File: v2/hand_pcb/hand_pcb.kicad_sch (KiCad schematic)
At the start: 60 parts, among them J1 Screw_Terminal_01x10, J10 8P8C, J2 Conn_01x08, J3 Conn_01x08, J4 Conn_01x02, J5 Conn_01x02, J9 Conn_02x02_Top_Bottom, M1 Motor_Servo_FB, M10 Motor_Servo_FB, M2 Motor_Servo_FB, M3 Motor_Servo_FB, M4 Motor_Servo_FB, M5 Motor_Servo_FB, M6 Motor_Servo_FB, M7 Motor_Servo_FB, M8 Motor_Servo_FB, M9 Motor_Servo_FB, Q1 Q_NMOS_GDS, Q2 Q_NMOS_GDS, Q3 Q_NMOS_GDS, Q4 Q_NMOS_GDS, Q5 Q_NMOS_GDS, U1 PCA9685PW, U2 MCP23017_SP, U4 ADS7830, U5 ADS7830

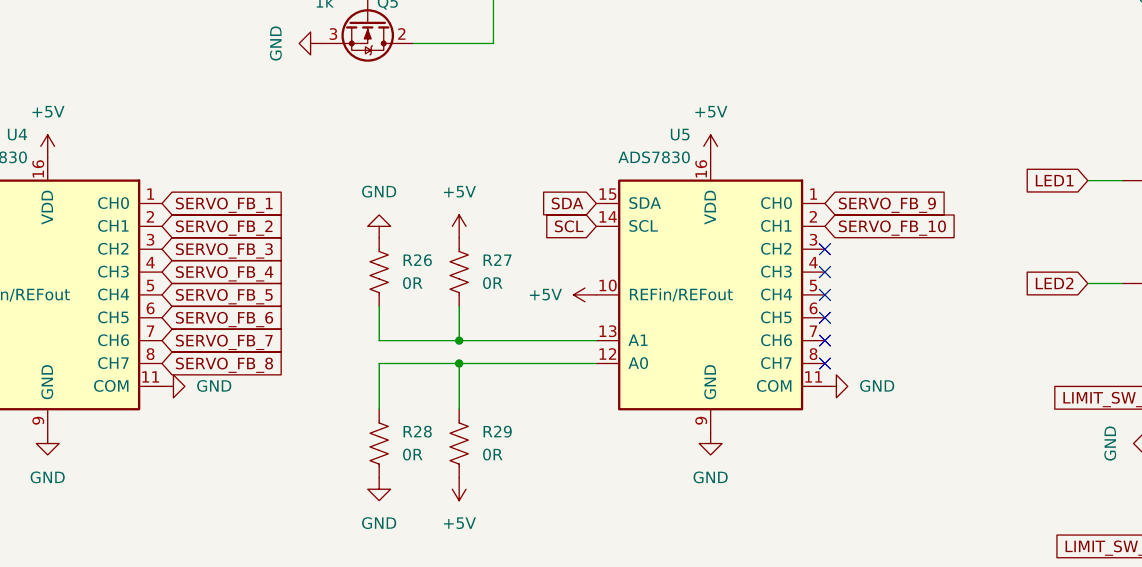
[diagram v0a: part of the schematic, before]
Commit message: Doing stuff
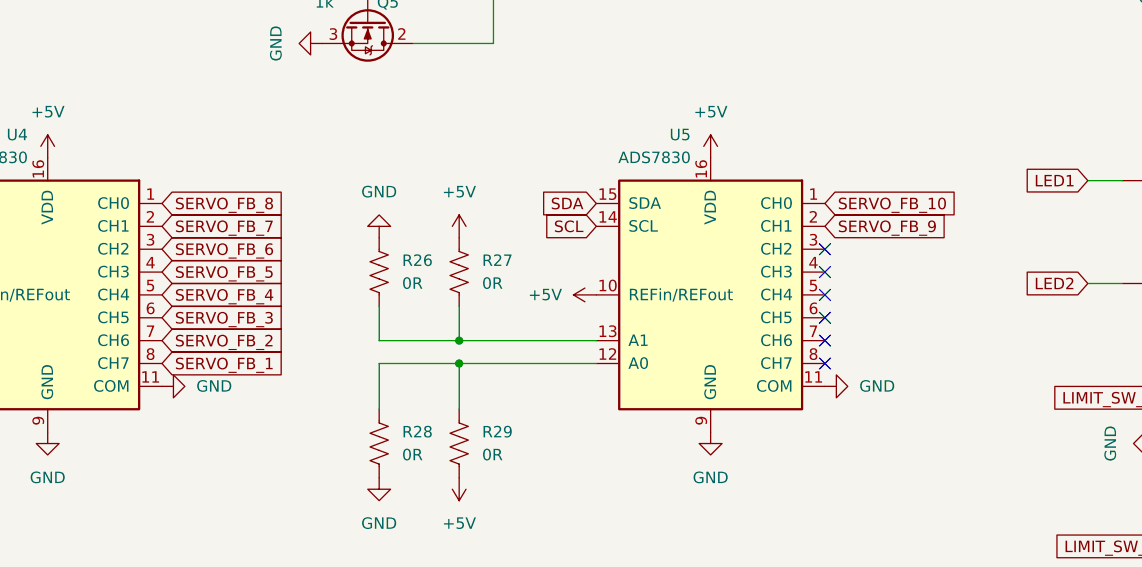
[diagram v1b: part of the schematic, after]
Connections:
- net SERVO_FB_1: now also U4.8 (CH7); no longer U4.1 (CH0)
- net SERVO_FB_10: now also U5.1 (CH0); no longer U5.2 (CH1)
- net SERVO_FB_2: now also U4.7 (CH6); no longer U4.2 (CH1)
- net SERVO_FB_3: now also U4.6 (CH5); no longer U4.3 (CH2)
- net SERVO_FB_4: now also U4.5 (CH4); no longer U4.4 (CH3)
- net SERVO_FB_5: now also U4.4 (CH3); no longer U4.5 (CH4)
- net SERVO_FB_6: now also U4.3 (CH2); no longer U4.6 (CH5)
- net SERVO_FB_7: now also U4.2 (CH1); no longer U4.7 (CH6)
- net SERVO_FB_8: now also U4.1 (CH0); no longer U4.8 (CH7)
- net SERVO_FB_9: now also U5.2 (CH1); no longer U5.1 (CH0)
